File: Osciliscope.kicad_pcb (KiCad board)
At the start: 2 copper layers, 51 x 102 mm, 62 parts, among them J1 Conn_01x09_Socket, J2 Conn_01x04_Socket, J3 U.FL, J4 Conn_01x04_Socket, J5 USB_C_Receptacle_USB2.0_14P, J6 Conn_01x02_MountingPin, J7 U.FL, SW1 RotaryEncoder_Switch, SW3 SW_Nidec_CAS-120A1, SW4 SW_Nidec_CAS-120A1, SW5 RotaryEncoder_Switch, SW6 RotaryEncoder_Switch, U1 MCP1700x-330xxMB, U2 ADC082S101, U3 IP2721, U4 AZ1084-5.0, U5 TLV9061xDBV, U7 TLV9061xDBV, U8 MCP4251-104E/ML-ND

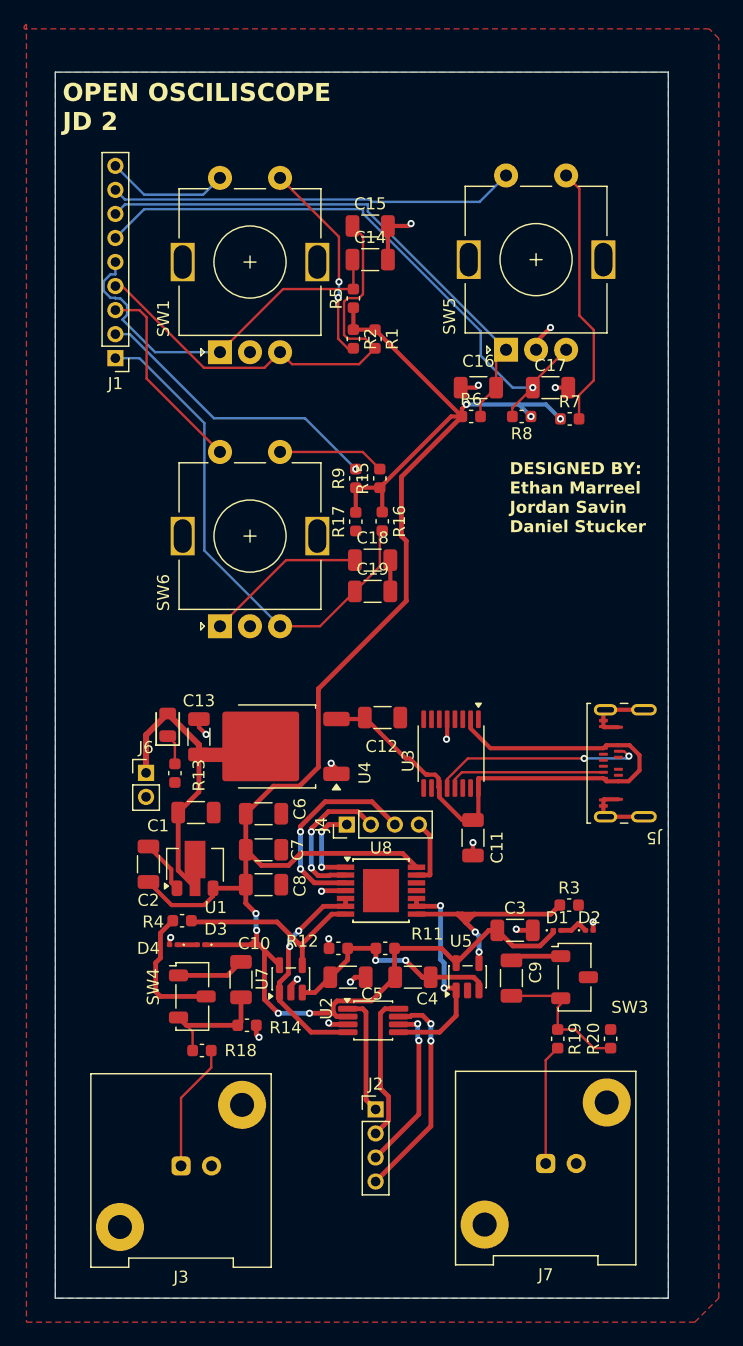
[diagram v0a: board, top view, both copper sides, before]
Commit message: DOUBLE POWAH
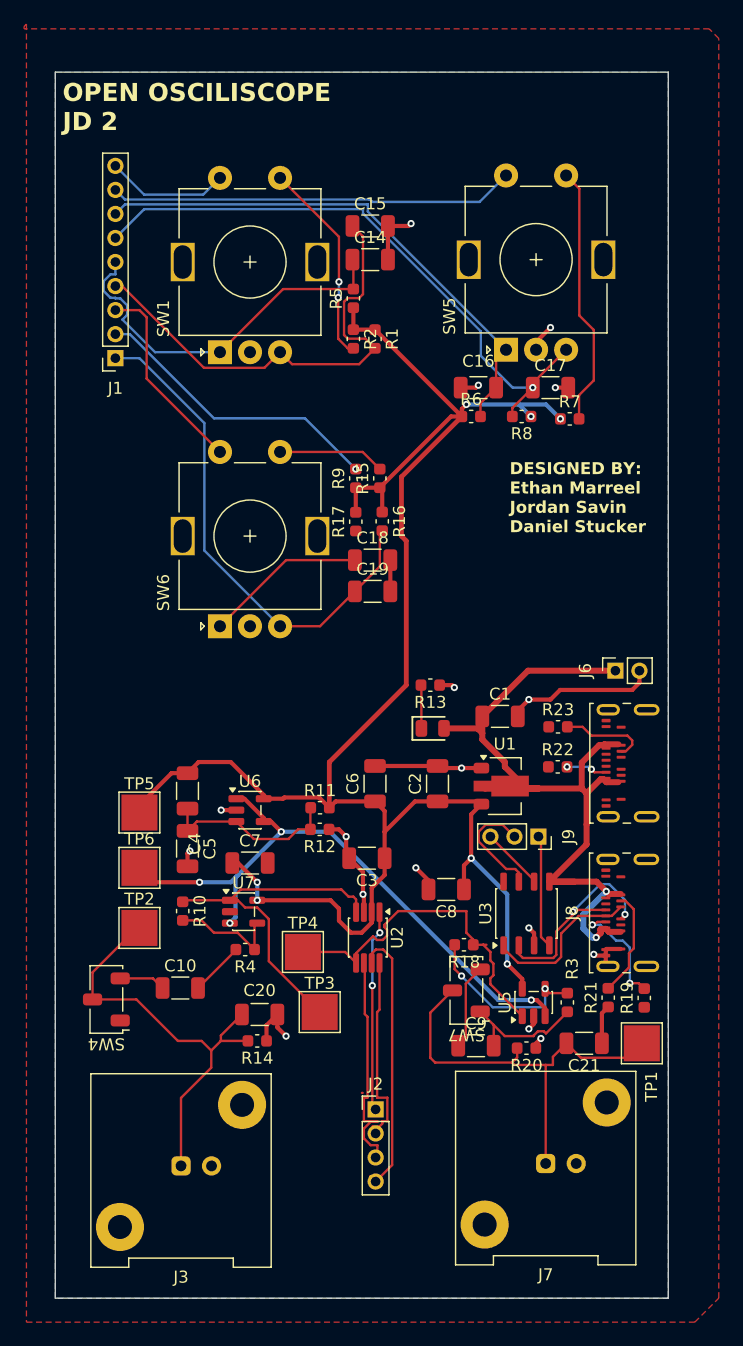
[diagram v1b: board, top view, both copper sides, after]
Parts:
- removed C11: 1uF, Capacitor_SMD:C_1206_3216Metric
- removed C12, C13: 10u, Capacitor_SMD:C_1206_3216Metric
- removed D1, D2, D3, D4: D, Diode_SMD:D_0201_0603Metric
- removed J4: Conn_01x04_Socket, Connector_PinHeader_2.00mm:PinHeader_1x04_P2.00mm_Vertical
- removed SW3: SW_Nidec_CAS-120A1, Button_Switch_SMD:Nidec_Copal_CAS-120A
- removed U4: AZ1084-5.0, Package_TO_SOT_SMD:TO-252-2
- removed U8: MCP4251-104E/ML-ND, Package_SO:TSSOP-14-1EP_4.4x5mm_P0.65mm
- added C20: 20pF, Capacitor_SMD:C_1206_3216Metric, F.Cu at (87.0, 168.4)
- added C21: 20pF, Capacitor_SMD:C_1206_3216Metric, F.Cu at (114.0, 170.8)
- added J8: USB_C_Receptacle_USB2.0_14P, Connector_USB:USB_C_Receptacle_Amphenol_124019772112A, F.Cu at (119.0, 159.9)
- added J9: Conn_01x03_Socket, Connector_PinSocket_2.00mm:PinSocket_1x03_P2.00mm_Vertical, F.Cu at (110.2, 153.6)
- added R10: 5k, Capacitor_SMD:C_0603_1608Metric, F.Cu at (80.6, 159.8)
- added R21: 5.5k, Capacitor_SMD:C_0603_1608Metric, F.Cu at (116.0, 167.0)
- added R22: 5.5k, Capacitor_SMD:C_0603_1608Metric, F.Cu at (111.8, 147.8)
- added R23: 5.5k, Capacitor_SMD:C_0603_1608Metric, F.Cu at (111.8, 144.5)
- added SW7: SW_Nidec_CAS-120A1, Button_Switch_SMD:Nidec_Copal_CAS-120A, F.Cu at (104.2, 166.4)
- added TP1: TestPoint, TestPoint:TestPoint_Pad_3.0x3.0mm, F.Cu at (118.8, 170.8)
- added TP2: TestPoint, TestPoint:TestPoint_Pad_3.0x3.0mm, F.Cu at (77.0, 161.2)
- added TP3: TestPoint, TestPoint:TestPoint_Pad_3.0x3.0mm, F.Cu at (92.0, 168.2)
- added TP4: TestPoint, TestPoint:TestPoint_Pad_3.0x3.0mm, F.Cu at (90.6, 163.2)
- added TP5: TestPoint, TestPoint:TestPoint_Pad_3.0x3.0mm, F.Cu at (77.0, 151.6)
- added TP6: TestPoint, TestPoint:TestPoint_Pad_3.0x3.0mm, F.Cu at (77.0, 156.2)
- added U6: TLV9061xDBV, Package_TO_SOT_SMD:SOT-23-5, F.Cu at (86.2, 151.4)
- J1: footprint Connector_PinHeader_2.00mm:PinHeader_1x09_P2.00mm_Vertical -> Connector_PinSocket_2.00mm:PinSocket_1x09_P2.00mm_Vertical
- J6: footprint Connector_PinHeader_2.00mm:PinHeader_1x02_P2.00mm_Vertical -> Connector_PinSocket_2.00mm:PinSocket_1x02_P2.00mm_Vertical
- R14, R20: value 100k -> 1M
- R18: value 1M -> 5k
- R19: value 1M -> 5.5k
- U3: value IP2721 -> CH340N; footprint Package_SO:TSSOP-16_4.4x5mm_P0.65mm -> Package_SO:JEITA_SOIC-8_3.9x4.9mm_P1.27mm
- moved J6 40.0 mm to (116.6, 139.8), turned to 90 degrees
- moved U1 26.6 mm to (107.4, 149.4), turned to 0 degrees
- moved C1 26.5 mm to (107.0, 143.6)
- moved C2 25.0 mm to (101.8, 149.2)
- moved C4 24.3 mm to (81.0, 149.8), turned to -90 degrees
- moved R18 23.5 mm to (104.0, 162.6), turned to 180 degrees
- moved R13 22.5 mm to (101.2, 141.0), turned to 180 degrees
- moved D5 22.1 mm to (101.4, 144.6), turned to 0 degrees
- moved C5 17.1 mm to (81.0, 154.6), turned to -90 degrees
- moved C8 15.2 mm to (102.5, 158.0), turned to 180 degrees
- moved U3 14.7 mm to (109.2, 160.0), turned to 90 degrees
- moved C3 13.7 mm to (95.9, 155.4), turned to 180 degrees
- moved R11 12.9 mm to (92.0, 151.2)
- moved R12 10.0 mm to (92.0, 153.0), turned to 180 degrees
- moved C6 9.61 mm to (96.6, 149.2), turned to 90 degrees
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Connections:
- net C2_G_IN renamed Net-(U7--)
- net C2_G_OUT renamed CHAN_2
- C4 pad 2: V1.8 -> V1.65RAW
- C5 pad 1: V1.8 -> V1.65RAW
- C9 pad 1: Net-(SW3-A) -> Net-(SW7-A)
- C9 pad 2: Net-(SW3-C) -> Net-(SW7-C)
- J5 pad A4: USBCRAW -> 5Vin
- J5 pad A9: USBCRAW -> 5Vin
- J5 pad B4: USBCRAW -> 5Vin
- J5 pad B9: USBCRAW -> 5Vin
- R11 pad 1: V1.8 -> V1.65RAW
- R12 pad 2: V1.8 -> V1.65RAW
- R14 pad 1: Net-(SW4-A) -> GND
- R14 pad 2: GND -> Net-(J3-In)
- R18 pad 1: Net-(SW4-A) -> CHAN_1
- R18 pad 2: Net-(J3-In) -> Net-(U5--)
- R19 pad 1: Net-(SW3-A) -> GND
- R19 pad 2: Net-(J7-In) -> Net-(J8-CC1)
- R20 pad 1: Net-(SW3-A) -> GND
- R20 pad 2: GND -> Net-(J7-In)
- R3 pad 1: C1_G_IN -> Net-(U5--)
- R3 pad 2: unconnected-(R3-Pad2) -> Net-(SW7-C)
- R4 pad 2: Net-(SW4-B) -> Net-(SW4-C)
- SW4 pad 2: Net-(SW4-B) -> Net-(J3-In)
- U2 pad 5: C1_G_OUT -> CHAN_1
- U3 pad 1: unconnected-(U3-VBUSG-Pad1) -> Net-(U3-UD+)
- U3 pad 2: USBCRAW -> Net-(U3-UD-)
- U3 pad 3: unconnected-(U3-NC-Pad3) -> GND
- U3 pad 4: unconnected-(U3-NC-Pad4) -> RTS
- U3 pad 5: GND -> 5Vin
- U3 pad 6: unconnected-(U3-NC-Pad6) -> TXD
- U3 pad 7: unconnected-(U3-NC-Pad7) -> RXD
- U5 pad 1: C1_G_OUT -> CHAN_1
- U5 pad 3: V1.8 -> V1.65
- U5 pad 4: C1_G_IN -> Net-(U5--)
- U7 pad 3: V1.8 -> V1.65
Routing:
- net V1.65: track 0.00 -> 52.6 mm, vias 0 -> 4
- net USBCRAW: track 51.3 -> 0.00 mm
- net 5Vin: track 22.5 -> 67.6 mm, vias 0 -> 2
- net CHAN_1: track 0.00 -> 29.0 mm
- net Net-(J7-In): track 10.0 -> 35.9 mm
- net Net-(J3-In): track 10.6 -> 36.1 mm
- net V1.8: track 19.2 -> 0.00 mm, vias 2 -> 0
- net C1_G_IN: track 19.2 -> 0.00 mm, vias 2 -> 0
- net GND: track 45.2 -> 64.3 mm
- net Net-(U3-UD-): track 0.00 -> 18.5 mm, vias 0 -> 2
- net C1_G_OUT: track 18.2 -> 0.00 mm, vias 2 -> 0
- net RPI_DIN_DP: track 17.3 -> 0.00 mm, vias 2 -> 0
- net V1.65RAW: track 0.00 -> 15.1 mm
- net Net-(U5--): track 0.00 -> 14.5 mm, vias 0 -> 2
- net Net-(U3-UD+): track 0.00 -> 13.6 mm
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
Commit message: Footprint updates
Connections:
- R3 pad 2: Net-(SW7-C) -> Net-(R3-Pad2)
- R4 pad 2: Net-(SW4-C) -> Net-(R4-Pad2)
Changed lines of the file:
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@@
 	(net 46 "Net-(SW7-C)")
 	(net 47 "V1.65RAW")
+	(net 48 "Net-(R3-Pad2)")
+	(net 49 "Net-(R4-Pad2)")
 	(footprint "Connector_USB:USB_C_Receptacle_Amphenol_124019772112A"
 		(layer "F.Cu")
@@
 			(layers "F.Cu" "F.Mask" "F.Paste")
 			(roundrect_rratio 0.25)
-			(net 46 "Net-(SW7-C)")
+			(net 48 "Net-(R3-Pad2)")
 			(pintype "passive")
 		)
@@
 			(layers "F.Cu" "F.Mask" "F.Paste")
 			(roundrect_rratio 0.25)
-			(net 9 "Net-(SW4-C)")
+			(net 49 "Net-(R4-Pad2)")
 			(pintype "passive")
 		)
